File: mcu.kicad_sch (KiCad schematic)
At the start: 23 parts, among them J1 USB4105-GF-A-120, U1 STM32G473CEUx, Y1 ECS-240-6-37B-7KM-TR

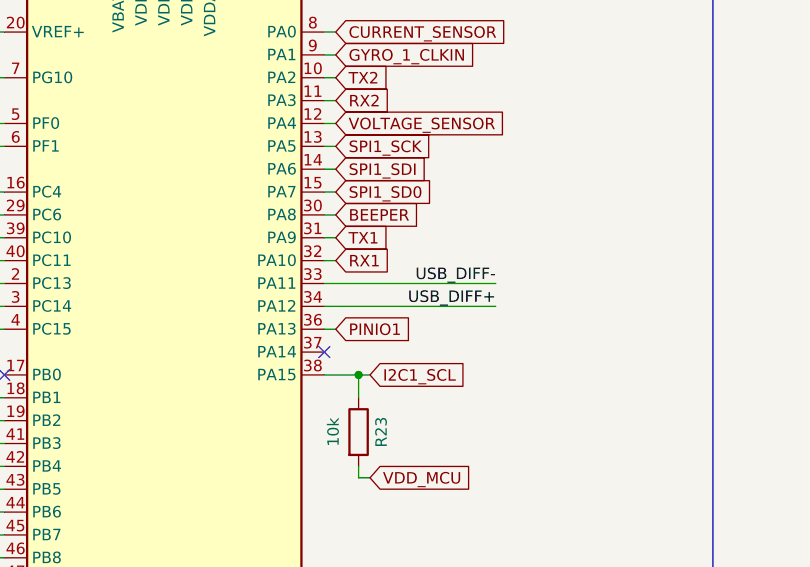
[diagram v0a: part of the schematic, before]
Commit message: routing
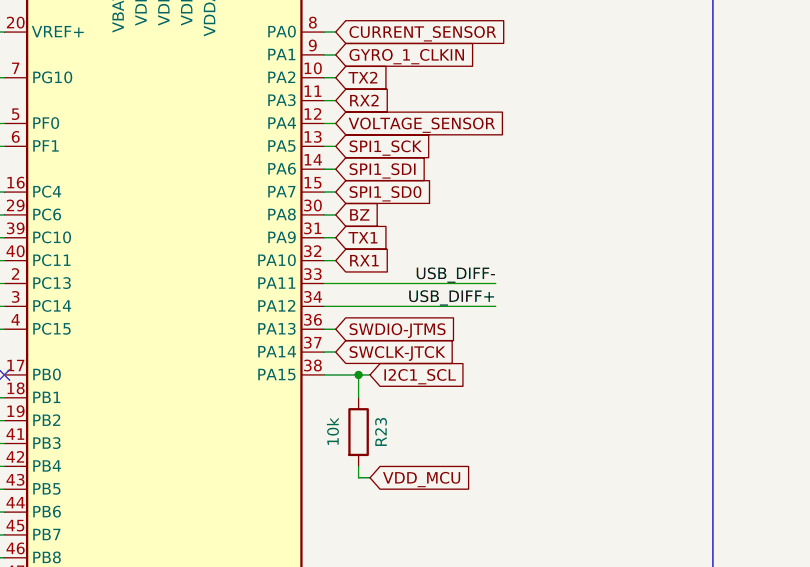
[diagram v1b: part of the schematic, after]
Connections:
- net SWCLK-JTCK: now reaches U1.37 (PA14)
- net BEEPER renamed BZ
- net PINIO1 renamed SWDIO-JTMS
- no-connect marks 4 -> 3
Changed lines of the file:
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@@
 		(at 234.95 106.68)
 	)
-	(no_connect
-		(at 116.84 123.19)
-	)
 	(wire
 		(pts
@@
 		(pts
 			(xy 58.42 146.05) (xy 81.28 146.05)
+		)
+		(stroke
+			(width 0)
+			(type default)
+		)
+	)
+	(wire
+		(pts
+			(xy 116.84 123.19) (xy 118.11 123.19)
 		)
 		(stroke
@@
 		)
 	)
-	(global_label "PINIO1"
+	(global_label "SPI1_SDI"
+		(shape input)
+		(at 118.11 102.87 0)
+		(fields_autoplaced yes)
+		(effects
+			(font
+				(size 1.27 1.27)
+			)
+			(justify left)
+		)
+		(property "Intersheetrefs" "${INTERSHEET_REFS}"
+			(at 129.4409 102.87 0)
+			(effects
+				(font
+					(size 1.27 1.27)
+				)
+				(justify left)
+				(hide yes)
+			)
+		)
+	)
+	(global_label "SWCLK-JTCK"
+		(shape input)
+		(at 118.11 123.19 0)
+		(fields_autoplaced yes)
+		(effects
+			(font
+				(size 1.27 1.27)
+			)
+			(justify left)
+		)
+		(property "Intersheetrefs" "${INTERSHEET_REFS}"
+			(at 133.3718 123.19 0)
+			(effects
+				(font
+					(size 1.27 1.27)
+				)
+				(justify left)
+				(hide yes)
+			)
+		)
+	)
+	(global_label "VDD_MCU"
+		(shape input)
+		(at 58.42 162.56 270)
+		(fields_autoplaced yes)
+		(effects
+			(font
+				(size 1.27 1.27)
+			)
+			(justify right)
+		)
+		(property "Intersheetrefs" "${INTERSHEET_REFS}"
+			(at 58.42 174.1933 90)
+			(effects
+				(font
+					(size 1.27 1.27)
+				)
+				(justify right)
+				(hide yes)
+			)
+		)
+	)
+	(global_label "SPI2_SD0"
+		(shape input)
+		(at 80.01 163.83 180)
+		(fields_autoplaced yes)
+		(effects
+			(font
+				(size 1.27 1.27)
+			)
+			(justify right)
+		)
+		(property "Intersheetrefs" "${INTERSHEET_REFS}"
+			(at 68.0744 163.83 0)
+			(effects
+				(font
+					(size 1.27 1.27)
+				)
+				(justify right)
+				(hide yes)
+			)
+		)
+	)
+	(global_label "BZ"
+		(shape input)
+		(at 118.11 107.95 0)
+		(fields_autoplaced yes)
+		(effects
+			(font
+				(size 1.27 1.27)
+			)
+			(justify left)
+		)
+		(property "Intersheetrefs" "${INTERSHEET_REFS}"
+			(at 123.5747 107.95 0)
+			(effects
+				(font
+					(size 1.27 1.27)
+				)
+				(justify left)
+				(hide yes)
+			)
+		)
+	)
+	(global_label "5V_USB"
+		(shape input)
+		(at 237.49 101.6 0)
+		(fields_autoplaced yes)
+		(effects
+			(font
+				(size 1.27 1.27)
+			)
+			(justify left)
+		)
+		(property "Intersheetrefs" "${INTERSHEET_REFS}"
+			(at 247.5509 101.6 0)
+			(effects
+				(font
+					(size 1.27 1.27)
+				)
+				(justify left)
+				(hide yes)
+			)
+		)
+	)
+	(global_label "TX3"
+		(shape input)
+		(at 80.01 151.13 180)
+		(fields_autoplaced yes)
+		(effects
+			(font
+				(size 1.27 1.27)
+			)
+			(justify right)
+		)
+		(property "Intersheetrefs" "${INTERSHEET_REFS}"
+			(at 73.6382 151.13 0)
+			(effects
+				(font
+					(size 1.27 1.27)
+				)
+				(justify right)
+				(hide yes)
+			)
+		)
+	)
+	(global_label "SWDIO-JTMS"
 		(shape input)
 		(at 118.11 120.65 0)
@@
 		)
 		(property "Intersheetrefs" "${INTERSHEET_REFS}"
-			(at 127.4453 120.65 0)
+			(at 133.1299 120.65 0)
 			(effects
 				(font
@@
 				(hide yes)
 			)
-		)
-	)
-	(global_label "SPI1_SDI"
-		(shape input)
-		(at 118.11 102.87 0)
-		(fields_autoplaced yes)
-		(effects
-			(font
-				(size 1.27 1.27)
-			)
-			(justify left)
-		)
-		(property "Intersheetrefs" "${INTERSHEET_REFS}"
-			(at 129.4409 102.87 0)
-			(effects
-				(font
-					(size 1.27 1.27)
-				)
-				(justify left)
-				(hide yes)
-			)
-		)
-	)
-	(global_label "VDD_MCU"
-		(shape input)
-		(at 58.42 162.56 270)
-		(fields_autoplaced yes)
-		(effects
-			(font
-				(size 1.27 1.27)
-			)
-			(justify right)
-		)
-		(property "Intersheetrefs" "${INTERSHEET_REFS}"
-			(at 58.42 174.1933 90)
-			(effects
-				(font
-					(size 1.27 1.27)
-				)
-				(justify right)
-				(hide yes)
-			)
-		)
-	)
-	(global_label "SPI2_SD0"
-		(shape input)
-		(at 80.01 163.83 180)
-		(fields_autoplaced yes)
-		(effects
-			(font
-				(size 1.27 1.27)
-			)
-			(justify right)
-		)
-		(property "Intersheetrefs" "${INTERSHEET_REFS}"
-			(at 68.0744 163.83 0)
-			(effects
-				(font
-					(size 1.27 1.27)
-				)
-				(justify right)
-				(hide yes)
-			)
-		)
-	)
-	(global_label "BEEPER"
-		(shape input)
-		(at 118.11 107.95 0)
-		(fields_autoplaced yes)
-		(effects
-			(font
-				(size 1.27 1.27)
-			)
-			(justify left)
-		)
-		(property "Intersheetrefs" "${INTERSHEET_REFS}"
-			(at 128.3522 107.95 0)
-			(effects
-				(font
-					(size 1.27 1.27)
-				)
-				(justify left)
-				(hide yes)
-			)
-		)
-	)
-	(global_label "5V_USB"
-		(shape input)
-		(at 237.49 101.6 0)
-		(fields_autoplaced yes)
-		(effects
-			(font
-				(size 1.27 1.27)
-			)
-			(justify left)
-		)
-		(property "Intersheetrefs" "${INTERSHEET_REFS}"
-			(at 247.5509 101.6 0)
-			(effects
-				(font
-					(size 1.27 1.27)
-				)
-				(justify left)
-				(hide yes)
-			)
-		)
-	)
-	(global_label "TX3"
-		(shape input)
-		(at 80.01 151.13 180)
-		(fields_autoplaced yes)
-		(effects
-			(font
-				(size 1.27 1.27)
-			)
-			(justify right)
-		)
-		(property "Intersheetrefs" "${INTERSHEET_REFS}"
-			(at 73.6382 151.13 0)
-			(effects
-				(font
-					(size 1.27 1.27)
-				)
-				(justify right)
-				(hide yes)
-			)
